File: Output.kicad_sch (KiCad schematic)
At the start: 46 parts, among them J20 Conn_01x02, J21 Conn_01x02, Q1 2N7002NXAK, Q10 SSM3K361TU,LF, Q11 SSM3K361TU,LF, Q2 NTR5105PT1G, Q3 NTR5105PT1G, Q4 SSM3K361TU,LF, Q5 SSM3K361TU,LF, Q6 2N7002NXAK, Q7 SSM3K361TU,LF, Q8 SSM3K361TU,LF, Q9 SSM3K361TU,LF

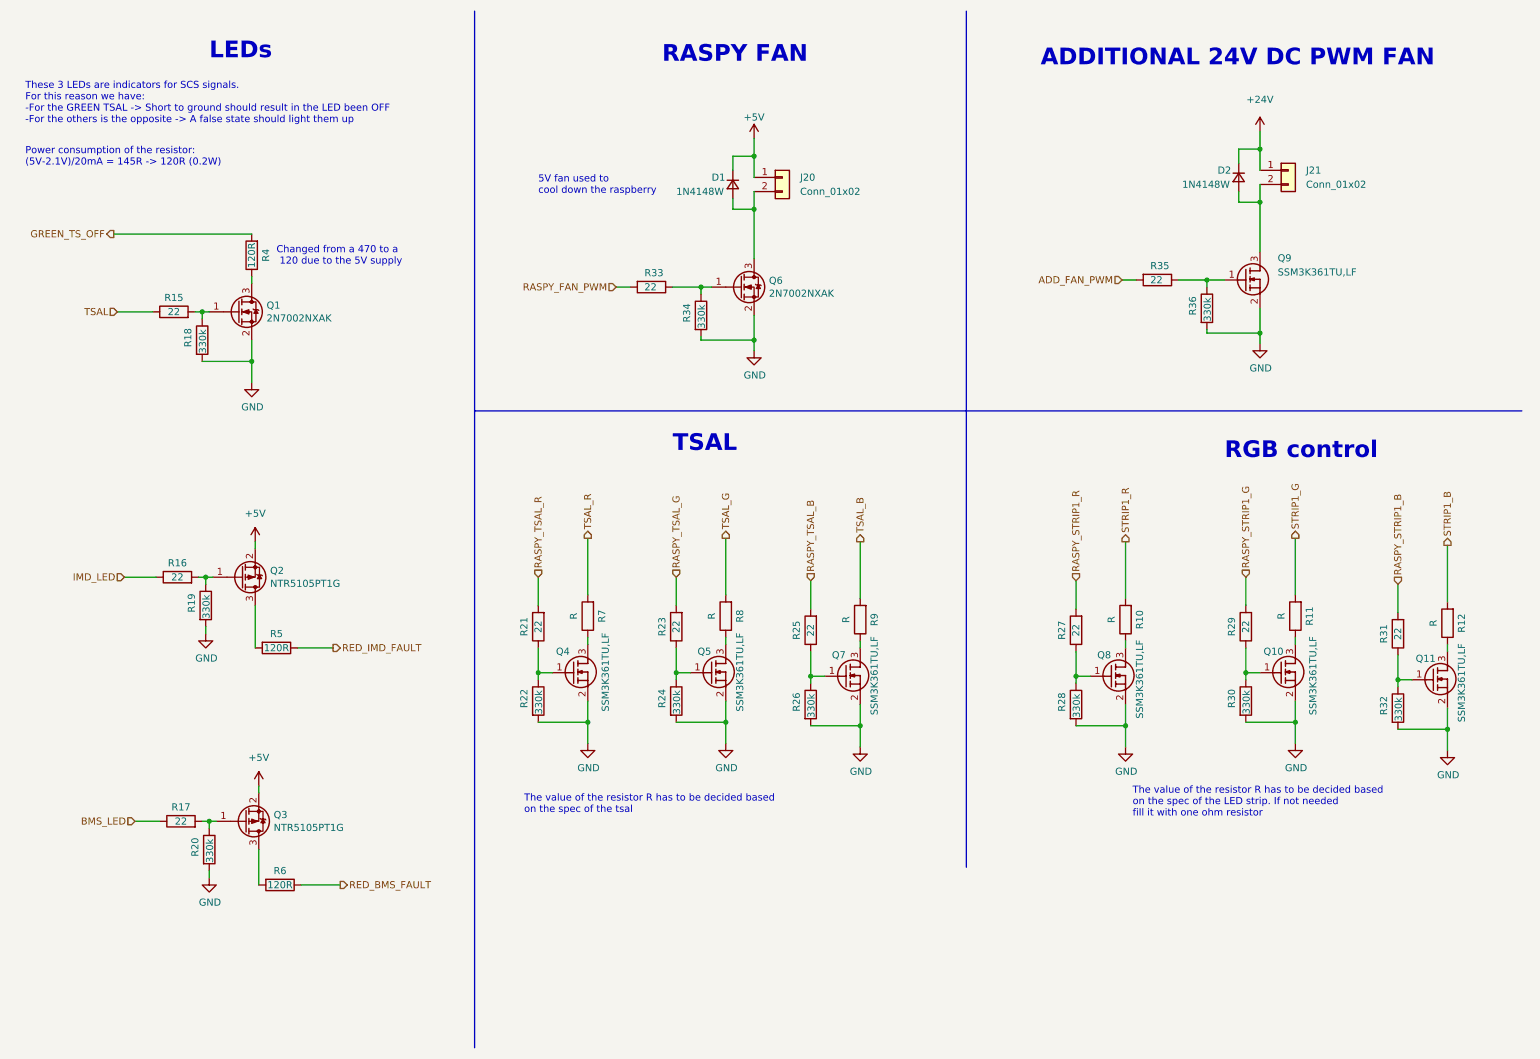
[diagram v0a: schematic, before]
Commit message: Major changes after the schematic review. Refer to Github for all the changes
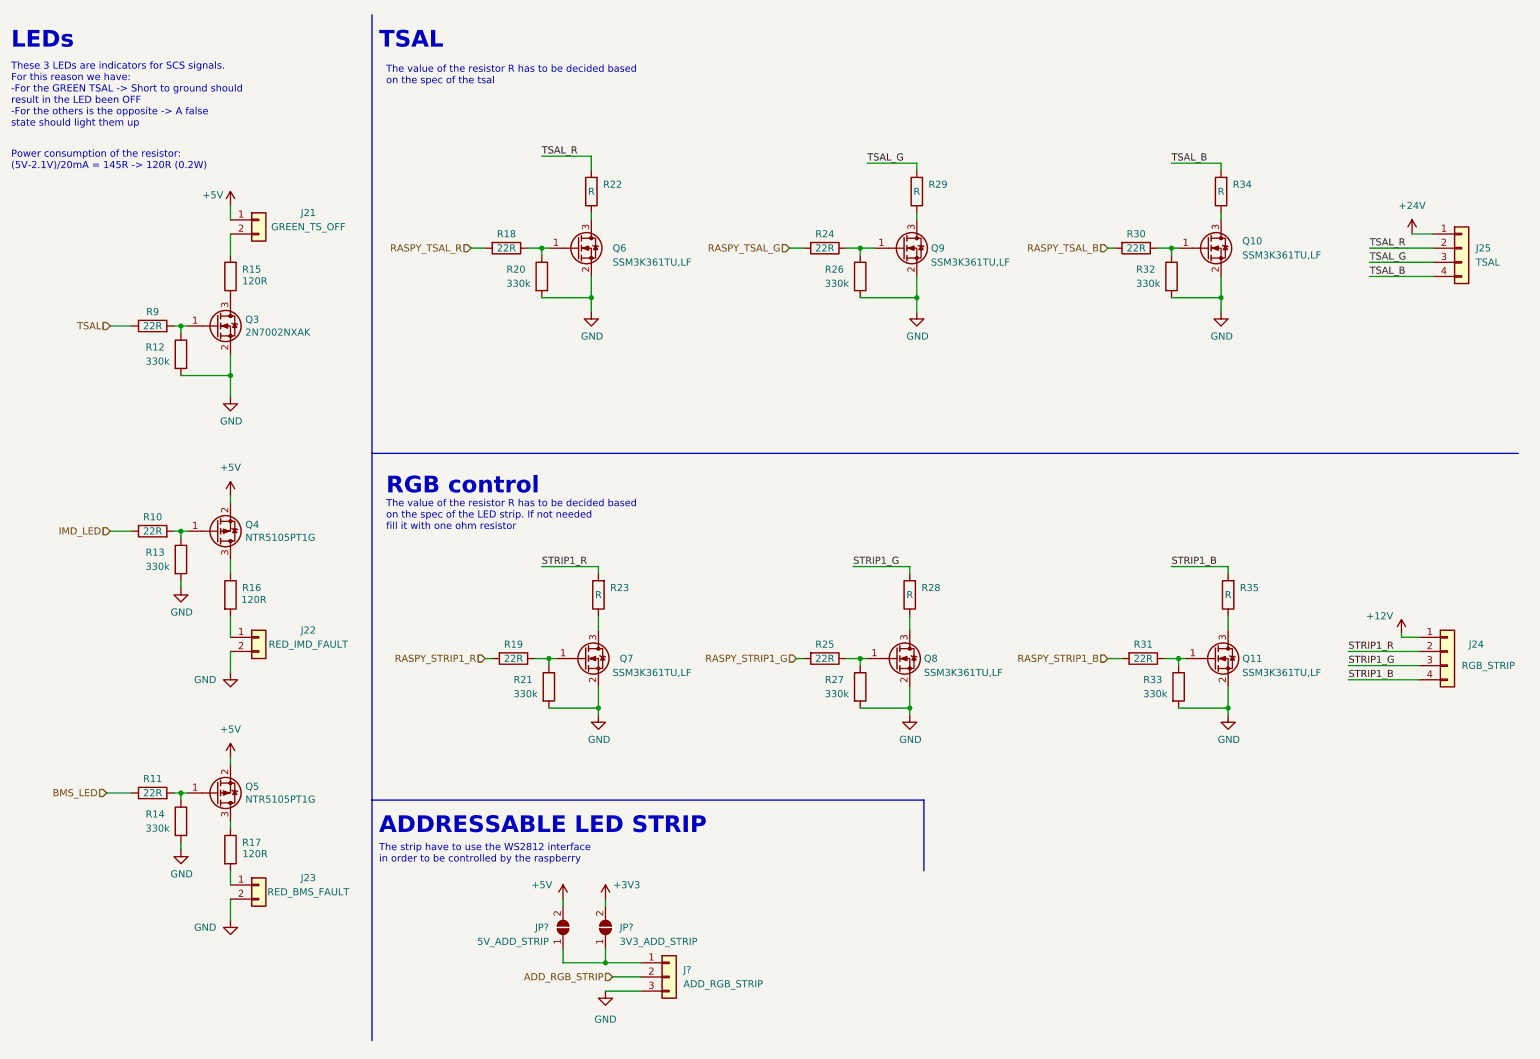
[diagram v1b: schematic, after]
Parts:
- removed D1, D2: 1N4148W, Diode_SMD:D_SOD-323_HandSoldering, symbol Device:D_Small
- removed J20: Conn_01x02, Connector_Molex:Molex_Micro-Fit_3.0_43650-0215_1x02_P3.00mm_Vertical, symbol Connector_Generic:Conn_01x02
- removed Q6: 2N7002NXAK, Package_TO_SOT_SMD:SOT-23, symbol Device:Q_NMOS_GSD
- removed Q9: SSM3K361TU,LF, 00_proj-lib:SOTFL65P210X75-3N, symbol 00_proj-lib:SSM3K361TU,LF
- removed R33, R35: 22, Resistor_SMD:R_0603_1608Metric, symbol Device:R
- removed R34, R36: 330k, Resistor_SMD:R_0603_1608Metric, symbol Device:R
- added J22: RED_IMD_FAULT, Connector_Molex:Molex_Micro-Fit_3.0_43650-0215_1x02_P3.00mm_Vertical, symbol Connector_Generic:Conn_01x02
- added J23: RED_BMS_FAULT, Connector_Molex:Molex_Micro-Fit_3.0_43650-0215_1x02_P3.00mm_Vertical, symbol Connector_Generic:Conn_01x02
- added J24: RGB_STRIP, Connector_Molex:Molex_Micro-Fit_3.0_43650-0400_1x04_P3.00mm_Horizontal, symbol Connector_Generic:Conn_01x04
- added J25: TSAL, Connector_Molex:Molex_Micro-Fit_3.0_43650-0400_1x04_P3.00mm_Horizontal, symbol Connector_Generic:Conn_01x04
- added J?: ADD_RGB_STRIP, Connector_Molex:Molex_Micro-Fit_3.0_43650-0315_1x03_P3.00mm_Vertical, symbol Connector_Generic:Conn_01x03
- added JP?: 5V_ADD_STRIP, symbol Jumper:SolderJumper_2_Open
- added JP?: 3V3_ADD_STRIP, symbol Jumper:SolderJumper_2_Open
- J21: value Conn_01x02 -> GREEN_TS_OFF
- Q10: renamed from Q7; symbol 00_proj-lib:SSM3K361TU,LF -> Device:Q_NMOS_GSD
- Q11: symbol 00_proj-lib:SSM3K361TU,LF -> Device:Q_NMOS_GSD
- Q6: renamed from Q4; symbol 00_proj-lib:SSM3K361TU,LF -> Device:Q_NMOS_GSD
- Q7: renamed from Q8; symbol 00_proj-lib:SSM3K361TU,LF -> Device:Q_NMOS_GSD
- Q8: renamed from Q10; symbol 00_proj-lib:SSM3K361TU,LF -> Device:Q_NMOS_GSD
- Q9: renamed from Q5; symbol 00_proj-lib:SSM3K361TU,LF -> Device:Q_NMOS_GSD
- R10: renamed from R16; value 22 -> 22R
- R11: renamed from R17; value 22 -> 22R
- R15: renamed from R4; footprint Resistor_SMD:R_2512_6332Metric -> Resistor_SMD:R_0603_1608Metric
- R16: renamed from R5; footprint Resistor_SMD:R_2512_6332Metric -> Resistor_SMD:R_0603_1608Metric
- R17: renamed from R6; footprint Resistor_SMD:R_2512_6332Metric -> Resistor_SMD:R_0603_1608Metric
- R18: renamed from R21; value 22 -> 22R
- R19: renamed from R27; value 22 -> 22R
- R22: renamed from R7; footprint Resistor_SMD:R_1206_3216Metric -> Resistor_SMD:R_0805_2012Metric
- R23: renamed from R10; footprint Resistor_SMD:R_1206_3216Metric -> Resistor_SMD:R_0805_2012Metric
- R24: renamed from R23; value 22 -> 22R
- R25: renamed from R29; value 22 -> 22R
- R28: renamed from R11; footprint Resistor_SMD:R_1206_3216Metric -> Resistor_SMD:R_0805_2012Metric
- R29: renamed from R8; footprint Resistor_SMD:R_1206_3216Metric -> Resistor_SMD:R_0805_2012Metric
- R30: renamed from R25; value 22 -> 22R
- R31: value 22 -> 22R
- R34: renamed from R9; footprint Resistor_SMD:R_1206_3216Metric -> Resistor_SMD:R_0805_2012Metric
- R35: renamed from R12; footprint Resistor_SMD:R_1206_3216Metric -> Resistor_SMD:R_0805_2012Metric
- R9: renamed from R15; value 22 -> 22R
- renumbered Q1 to Q3, Q2 to Q4, Q3 to Q5, R18 to R12, R19 to R13, R20 to R14, R22 to R20, R28 to R21, R24 to R26, R30 to R27, R26 to R32, R32 to R33
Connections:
- net GREEN_TS_OFF is gone; now on an unnamed net: R15.2
- net RED_BMS_FAULT is gone; now on an unnamed net: R17.1
- net RED_IMD_FAULT is gone; now on an unnamed net: R16.1
- net +24V: now also J25.1 (Pin_1); no longer J21.1 (Pin_1)
- net +5V: now also J21.1 (Pin_1), JP?.2 (B)
- net GND: now also J22.2 (Pin_2), J23.2 (Pin_2), J?.3 (Pin_3)
- net STRIP1_B: now also J24.4 (Pin_4)
- net STRIP1_G: now also J24.3 (Pin_3)
- net STRIP1_R: now also J24.2 (Pin_2)
- net TSAL_B: now also J25.4 (Pin_4)
- net TSAL_G: now also J25.3 (Pin_3)
- net TSAL_R: now also J25.2 (Pin_2)
- net at Q5.3 (D): no longer R17.2
- net at Q4.3 (D): no longer R16.2
- new net: J?.1 (Pin_1), JP?.1 (A), JP?.1 (A)
- new net: J23.1 (Pin_1), R17.2
- new net: J22.1 (Pin_1), R16.2
- new net +12V: J24.1 (Pin_1)
- new net +3V3: JP?.2 (B)
- new net ADD_RGB_STRIP: J?.2 (Pin_2)
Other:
- note added: "ADDRESSABLE LED STRIP"
- note added: "The strip have to use the WS2812 interface in order to be controlled by the raspberry"
- note removed: "5V fan used to cool down the raspberry"
- note removed: "ADDITIONAL 24V DC PWM FAN"
- note removed: "Changed from a 470 to a 120 due to the 5V supply"
- note removed: "RASPY FAN"
- moved on the sheet: Q3, Q4, Q5, R10, R11, R12, R13, R14, R15, R16, R17, R18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
